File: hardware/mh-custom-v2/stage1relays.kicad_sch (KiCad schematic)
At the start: 14 parts, among them T3 AO3400A, T4 AO3400A

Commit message: laptop back, coordinating efforts
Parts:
- PS1: footprint CFM06S050-E - Cincon:CFM06S050E -> VB05-T2S05-E fromEasyEDA:VB05-T2S05-E
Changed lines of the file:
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@@
     (property "Reference" "PS1" (id 0) (at 87.63 151.13 0))
     (property "Value" "CFM06S050" (id 1) (at 87.63 153.67 0))
-    (property "Footprint" "CFM06S050-E - Cincon:CFM06S050E" (id 2) (at 97.79 156.21 0)
+    (property "Footprint" "VB05-T2S05-E fromEasyEDA:VB05-T2S05-E" (id 2) (at 97.79 156.21 0)
       (effects (font (size 1.27 1.27)) (justify left) hide)
     )

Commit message: added linear regulator for 3.3V peripherals and ADE7953 reset jumper
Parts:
- PS1: footprint VB05-T2S05-E fromEasyEDA:VB05-T2S05-E -> CFM06S050-E - Cincon:CFM06S050E
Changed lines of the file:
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@@
     (property "Reference" "PS1" (id 0) (at 87.63 151.13 0))
     (property "Value" "CFM06S050" (id 1) (at 87.63 153.67 0))
-    (property "Footprint" "VB05-T2S05-E fromEasyEDA:VB05-T2S05-E" (id 2) (at 97.79 156.21 0)
+    (property "Footprint" "CFM06S050-E - Cincon:CFM06S050E" (id 2) (at 97.79 156.21 0)
       (effects (font (size 1.27 1.27)) (justify left) hide)
     )

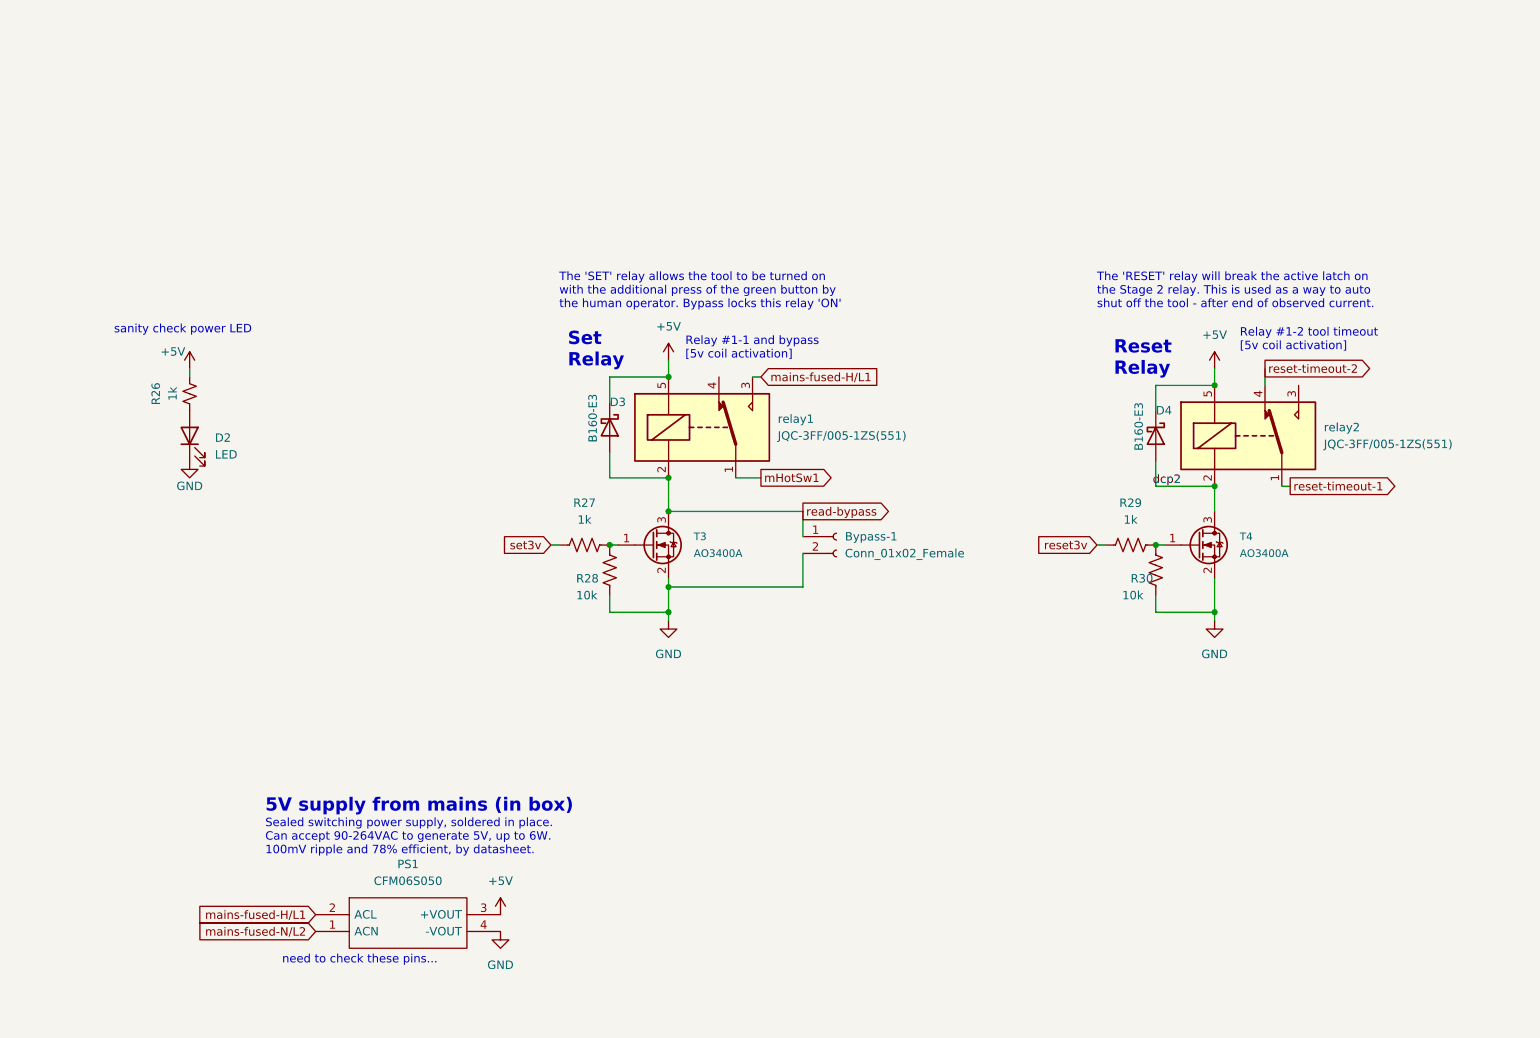
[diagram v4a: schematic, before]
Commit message: just ordered from JLCPCB
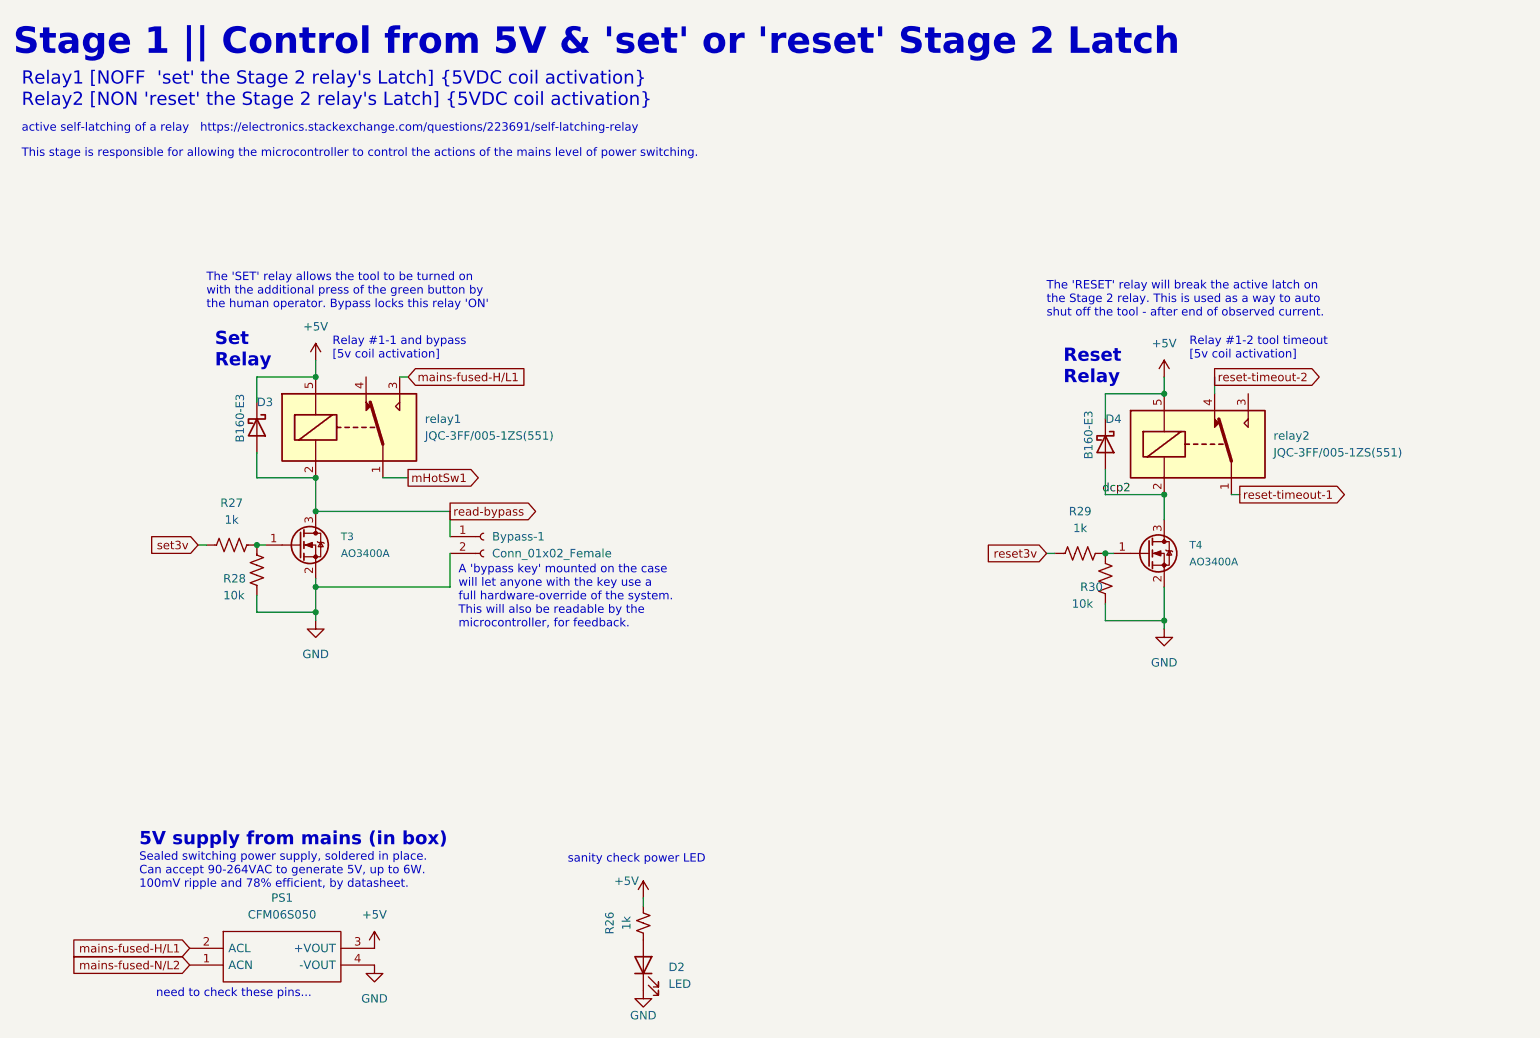
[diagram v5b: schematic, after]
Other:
- note added: "A 'bypass key' mounted on the case will let anyone with the key use a full hardware-override of the system. This will also be readable by the microcontroller, for feedback."
- note added: "Relay1 [NOFF 'set' the Stage 2 relay's Latch] {5VDC coil activation} Relay2 [NON 'reset' the Stage 2 relay's Latch] {5VDC coil activation}"
- note added: "Stage 1 || Control from 5V & 'set' or 'reset' Stage 2 Latch"
- note added: "This stage is responsible for allowing the microcontroller to control the actions of the mains level of power switching."
- note added: "active self-latching of a relay https://electronics.stackexchange.com/questions/223691/self-latching-relay"
- company: (none) -> Corey Rice & MakeHaven
- moved on the sheet: Bypass-1, D2, D3, D4, PS1, R26, R27, R28, R29, R30, T3, T4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
